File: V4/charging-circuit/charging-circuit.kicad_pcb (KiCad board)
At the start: 2 copper layers, 48.8 x 127.4 mm, 159 parts, among them CN1 DC3-2.54-14PAL, Q1 DMN2004K-7, Q11 BSS84, Q14 2N7002, Q17 CJQ4435, Q18 CJQ4435, Q2 DMN2004K-7, Q21 2N7002, Q22 CJQ4435, Q23 currentmirror, Q24 2N7002, Q25 2N7002, Q26 2N7002, Q27 CJQ4435, Q28 CJQ4435, Q3 DMN2004K-7, Q5 AO4892, SW3 TS-1088R-02026, U1 IP2326, U10 MAX3232CDBR, U12 ADS1115IDGSR, U19 TPL5110DDCT, U2 MAX17048G+T10, U3 BQ7692003PWR, U4 LM2596SX-3.3, U6 LM2596SX-5.0/NOPB, U7 2.54-2*20

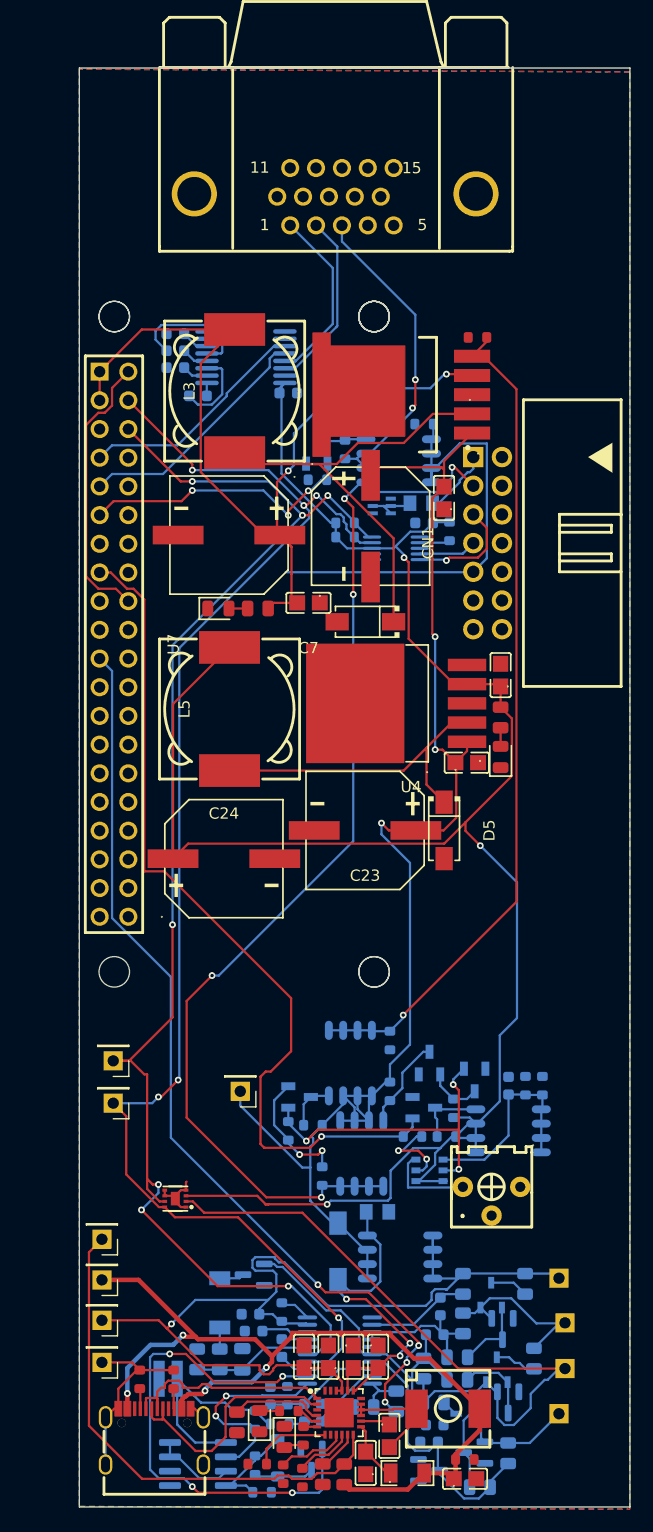
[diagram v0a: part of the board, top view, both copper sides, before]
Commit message: finished
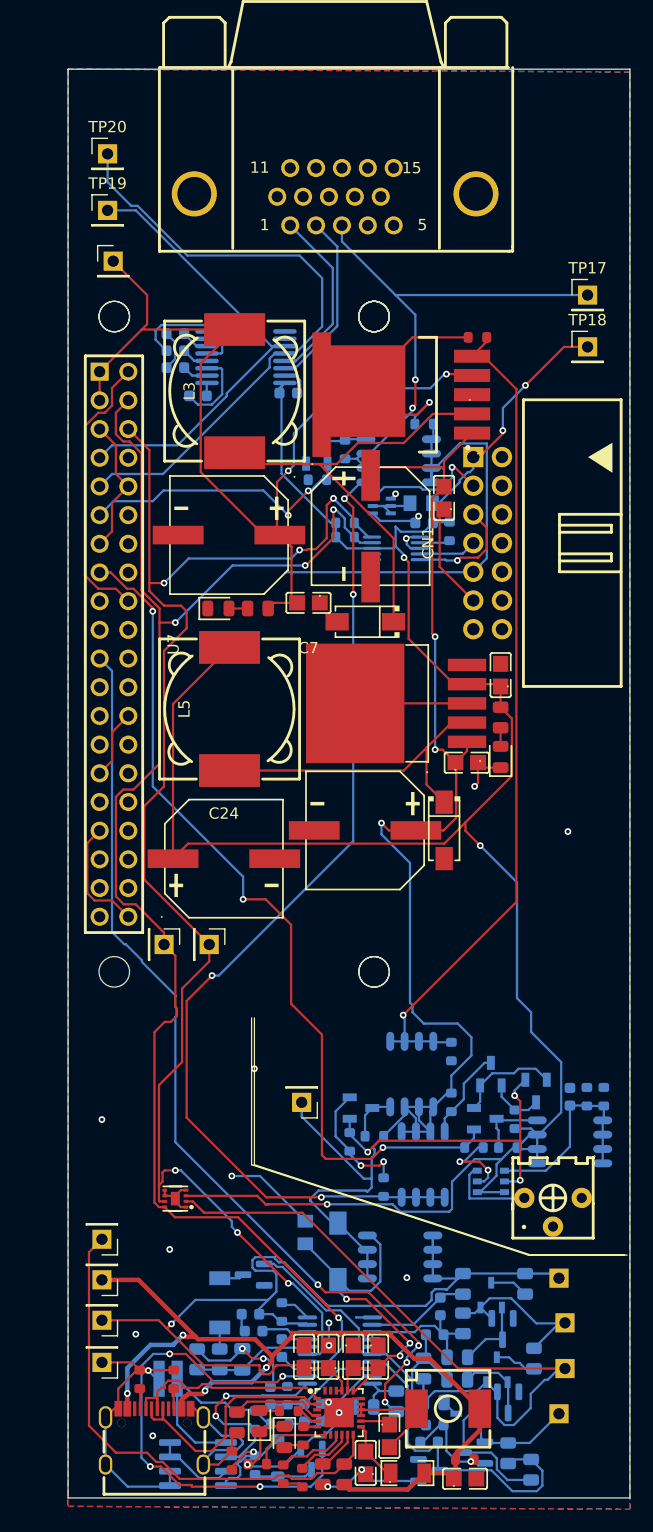
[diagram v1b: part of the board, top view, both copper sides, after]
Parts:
- removed the ? at (88.2, 132.0)
- removed the ? at (118.7, 132.0)
- removed the ? at (98.4, 132.0)
- added ?: , , F.Cu at (118.5, 132.0)
- added ?: , , F.Cu at (98.0, 132.0)
- added ?: , , F.Cu at (88.0, 132.0)
- added TP17: 12VOUT, Connector_PinHeader_2.54mm:PinHeader_1x01_P2.54mm_Vertical, F.Cu at (119.0, 68.5)
- added TP18: 3V3, Connector_PinHeader_2.54mm:PinHeader_1x01_P2.54mm_Vertical, F.Cu at (119.0, 73.1)
- added TP19: TX, Connector_PinHeader_2.54mm:PinHeader_1x01_P2.54mm_Vertical, F.Cu at (76.5, 61.0)
- added TP20: RX, Connector_PinHeader_2.54mm:PinHeader_1x01_P2.54mm_Vertical, F.Cu at (76.5, 56.0)
- added TP21: 5V, Connector_PinHeader_2.54mm:PinHeader_1x01_P2.54mm_Vertical, F.Cu at (77.0, 65.5)
- R54: moved to F.Cu
- moved TP15 14.8 mm to (81.5, 126.0), turned to -90 degrees
- moved TP16 13.4 mm to (85.5, 126.0), turned to -90 degrees
- moved R5 6.66 mm to (94.0, 151.5), turned to -90 degrees
- moved Q21 5.52 mm to (109.9, 141.4)
- moved R6 5.52 mm to (115.9, 149.7)
- moved C65 5.52 mm to (117.4, 139.5)
- moved Q22 5.52 mm to (117.4, 143.5)
- moved Q24 5.52 mm to (114.4, 139.0)
- moved Q25 5.52 mm to (98.9, 140.5)
- moved Q26 5.52 mm to (110.4, 137.5)
- moved Q27 5.52 mm to (103.4, 137.5)
- moved Q28 5.52 mm to (104.4, 145.5)
- moved R37 5.52 mm to (120.4, 139.5)
- moved R38 5.52 mm to (97.9, 143.5)
- moved R41 5.52 mm to (108.9, 144.0)
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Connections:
- C10 pad 2: /3S IC/ICGND -> /GND
- C11 pad 1: /3S IC/ICGND -> /GND
- C12 pad 2: /3S IC/ICGND -> /GND
- C16 pad 2: /3S Balancer/GND -> /GND
- C18 pad 1: /3S Balancer/GND -> /GND
- C27 pad 2: /3S Balancer/GND -> /GND
- C38 pad 2: /3S Balancer/GND -> /GND
- C39 pad 1: Net-(U3-VC0) -> Net-(U3-CAP1)
- C39 pad 2: Net-(U3-VC4) -> Net-(U3-VSS)
- C4 pad 1: /3S IC/ICGND -> /GND
- C40 pad 1: Net-(U3-SRP) -> Net-(U3-REGOUT)
- C40 pad 2: /3S Balancer/GND -> /GND
- C5 pad 1: /3S IC/ICGND -> /GND
- C8 pad 2: /3S IC/ICGND -> /GND
- C_sense7 pad 1: /3S Balancer/GND -> /GND
- C_sense9 pad 2: /3S Balancer/GND -> /GND
- D14 pad 1: /3S Balancer/GND -> /GND
- D8 pad 1: /3S IC/ICGND -> /GND
- D9 pad 1: /3S IC/ICGND -> /GND
- Q11 pad 1: /3S Balancer/GND -> /GND
- Q5 pad 5: /3S IC/ICGND -> /GND
- Q5 pad 6: /3S IC/ICGND -> /GND
- R12 pad 1: /3S IC/ICGND -> /GND
- R14 pad 1: Net-(U3-BAT) -> Net-(U3-ALERT)
- R14 pad 2: /3S Balancer/GND -> /GND
- R18 pad 1: /3S IC/ICGND -> /GND
- R22 pad 2: Net-(U3-BAT) -> Net-(U3-ALERT)
- R25 pad 2: /3S Balancer/GND -> /GND
- R31 pad 1: /3S IC/ICGND -> /GND
- R32 pad 1: /3S IC/ICGND -> /GND
- R33 pad 1: /3S IC/ICGND -> /GND
- R54 pad 2: /3S IC/ICGND -> /GND
- RPROG11 pad 2: /3S IC/ICGND -> /GND
- RPROG14 pad 2: /3S IC/ICGND -> /GND
- RPROG15 pad 2: /3S IC/ICGND -> /GND
- R_sense6 pad 2: /3S Balancer/GND -> /GND
- R_sense7 pad 2: Net-(U3-ALERT) -> Net-(U3-BAT)
- Rsense3 pad 2: /3S Balancer/GND -> /GND
- TP6 pad 1: /3S IC/ICGND -> /GND
- U1 pad 18: /3S IC/ICGND -> /GND
- U1 pad 25: /3S IC/ICGND -> /GND
- U3 pad 1: unconnected-(U3-DSG-Pad1) -> /3S Balancer/DSG
- U3 pad 11: /3S Balancer/DSG -> unconnected-(U3-NC-Pad11)
- U3 pad 12: /3S Balancer/CHG -> /3S Balancer/VC5
- U3 pad 13: Net-(U3-VC4) -> /3S Balancer/VC3
- U3 pad 14: /GPIO2/SDA1 -> /3S Balancer/VC3
- U3 pad 15: /GPIO3/SCL1 -> /3S Balancer/VC3
- U3 pad 16: /3S Balancer/TS1 -> /3S Balancer/VC1
- U3 pad 17: Net-(U3-VC0) -> /3S Balancer/VC0
- U3 pad 18: Net-(U3-SRP) -> /3S Balancer/SRP
- U3 pad 19: /3S IC/BAT+ -> /3S Balancer/SRN
- U3 pad 2: /3S Balancer/VC5 -> /3S Balancer/CHG
- U3 pad 3: /3S Balancer/VC3 -> Net-(U3-VSS)
- U3 pad 4: /3S Balancer/VC3 -> /GPIO2/SDA1
- U3 pad 5: /3S Balancer/VC3 -> /GPIO3/SCL1
- U3 pad 6: /3S Balancer/VC1 -> /3S Balancer/TS1
- U3 pad 7: /3S Balancer/VC0 -> Net-(U3-CAP1)
- U3 pad 8: /3S Balancer/SRP -> Net-(U3-REGOUT)
- U3 pad 9: /3S Balancer/SRN -> /3S IC/BAT+
- USBC1 pad 1: /3S IC/ICGND -> /GND
- USBC1 pad 2: /3S IC/ICGND -> /GND
- USBC1 pad 3: /3S IC/ICGND -> /GND
- USBC1 pad 4: /3S IC/ICGND -> /GND
- USBC1 pad A1B12: /3S IC/ICGND -> /GND
- USBC1 pad B1A12: /3S IC/ICGND -> /GND
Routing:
- net /GND: track 23.3 -> 226.6 mm, vias 4 -> 28
- net /GPIO15/RXD0: track 21.7 -> 55.3 mm
- net /DSUB+RS232/DSUB3.3V: track 191.2 -> 215.6 mm, vias 3 -> 5
- net /DSUB+RS232/DSUB12V: track 114.9 -> 136.3 mm
- net /GPIO14/TXD0: track 20.6 -> 41.3 mm
- net /3S IC/ICGND: track 18.1 -> 0.00 mm
- net /LM2596 3V3 BUCK/LM2596_VIN: track 122.7 -> 131.6 mm
- net /5V: track 77.8 -> 85.3 mm
- net /3S Balancer/VC0: track 23.8 -> 30.3 mm
- net /GPIO2/SDA1: track 128.0 -> 132.6 mm, vias 6 -> 4
- net Net-(Q3-G): track 8.31 -> 12.6 mm
- net Net-(U3-SRP): track 4.15 -> 0.00 mm
- net Net-(U3-REGOUT): track 0.00 -> 4.15 mm
- net Net-(U3-VSS): track 0.00 -> 2.70 mm
- net Net-(U3-VC4): track 2.70 -> 0.00 mm
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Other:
- board size 48.8 x 127.4 mm -> 49.8 x 126.5 mm
